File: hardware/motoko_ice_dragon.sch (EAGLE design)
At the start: 119 parts, among them IC2 LM2937, Q1 8MHz, Q10 20mA/30V, Q11 20mA/30V, Q2 BSS138TOP, Q3 BSS138TOP, Q4 20mA/30V, Q5 20mA/30V, Q6 20mA/30V, Q7 20mA/30V, Q8 20mA/30V, Q9 20mA/30V, U1 MP6540HA, U2 STM32_STM32F722XX, U3 MP6540HA

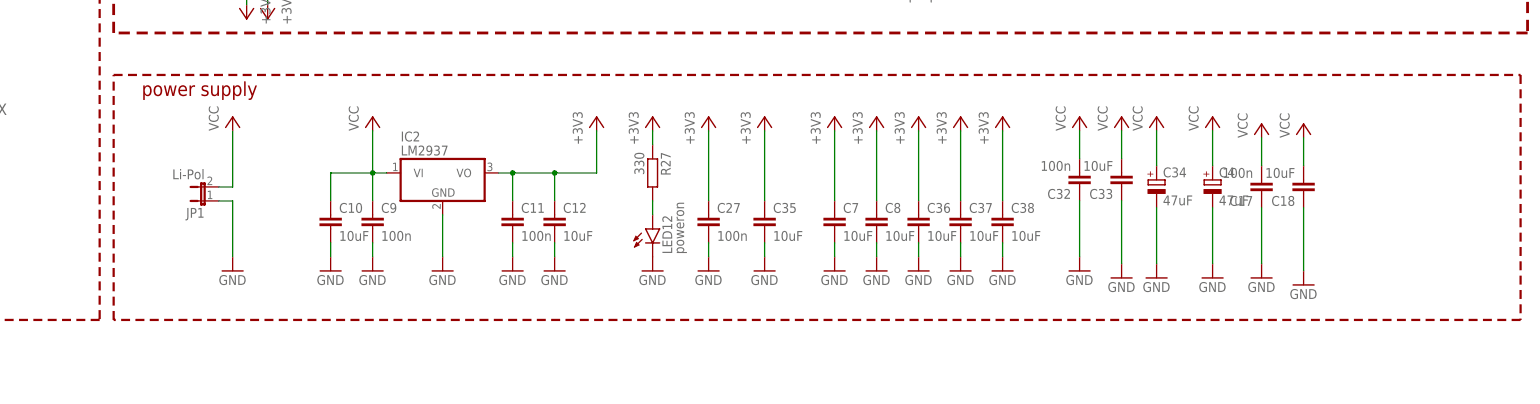
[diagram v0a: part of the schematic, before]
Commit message: main board
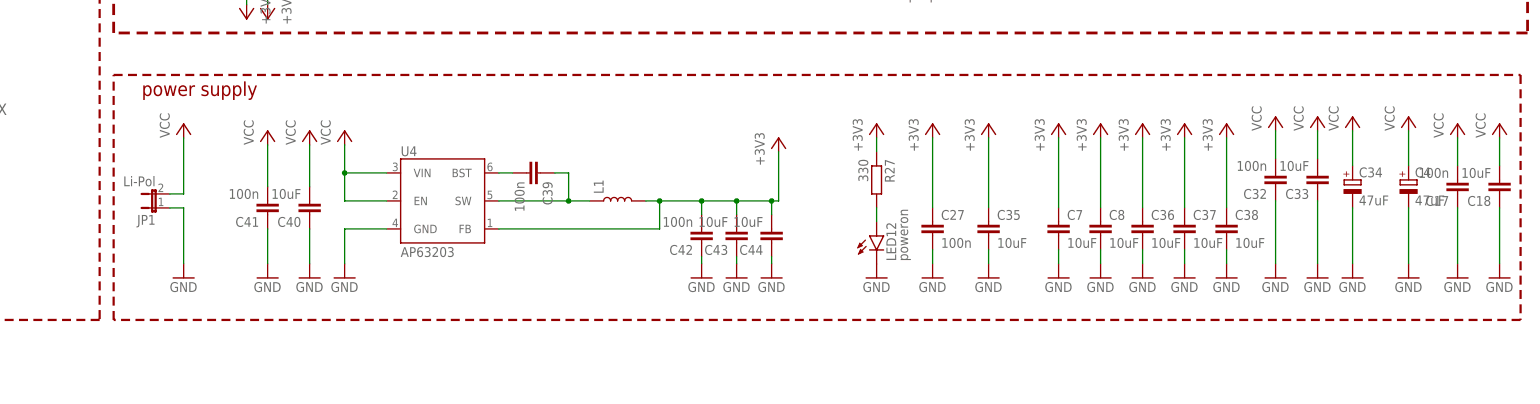
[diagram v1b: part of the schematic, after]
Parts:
- removed C10, C12: 10uF, resistor:C-EUC0805
- removed C11, C9: 100n, resistor:C-EUC0805
- removed IC2: LM2937, linear:LM2937
- added C39, C41, C42: 100n, resistor:C-EUC0805
- added C40, C43, C44: 10uF, resistor:C-EUC0805
- added L1: 4.7uH, TYS50204R7N-10, SparkFun-Coils:INDUCTOR-CR54-3.3UH
- added U4: AP63203, SparkFun-IC-Power:AP63203
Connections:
- new net N$22: C39.2, U4.BST
- new net N$26: C39.1, L1.1, U4.SW
- net +3V3: now also C42.2, C43.2, C44.2, L1.2, U4.FB; no longer C11.1, C12.1, IC2.VO
- net GND: now also C40.1, C41.1, C42.1, C43.1, C44.1, U4.GND; no longer C10.2, C11.2, C12.2, C9.2, IC2.GND
- net VCC: now also C40.2, C41.2, U4.EN, U4.VIN; no longer C10.1, C9.1, IC2.VI
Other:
- moved on the sheet: C17, C18, C27, C32, C33, C34, C35, C36, C37, C38, C4, C7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
